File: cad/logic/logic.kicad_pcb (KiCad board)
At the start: 2 copper layers, 93 x 60 mm, 36 parts, among them J1 Conn_01x02, J10 Conn_01x02, J2 Conn_01x02, J3 Conn_01x02, J4 Conn_01x02, J5 Conn_01x02, J6 Conn_01x02, J7 Conn_01x02, J8 Conn_01x02, J9 Conn_01x06, M3 MountingHole_3.2mm_M3_ISO7380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, U1 74HC595, U2 TPL7407LAD, U3 TPL7407LAD, U4 TPL7407LAD

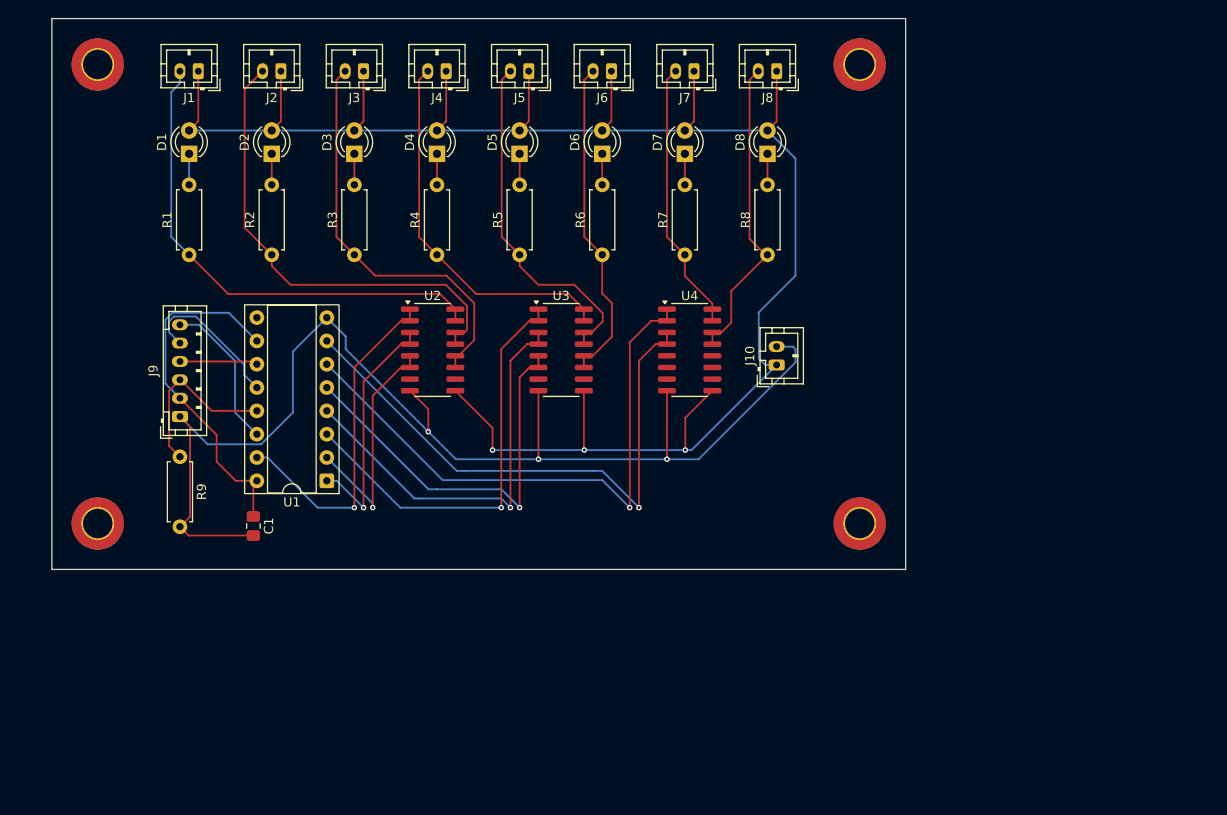
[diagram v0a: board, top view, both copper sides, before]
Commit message: Initial design complete
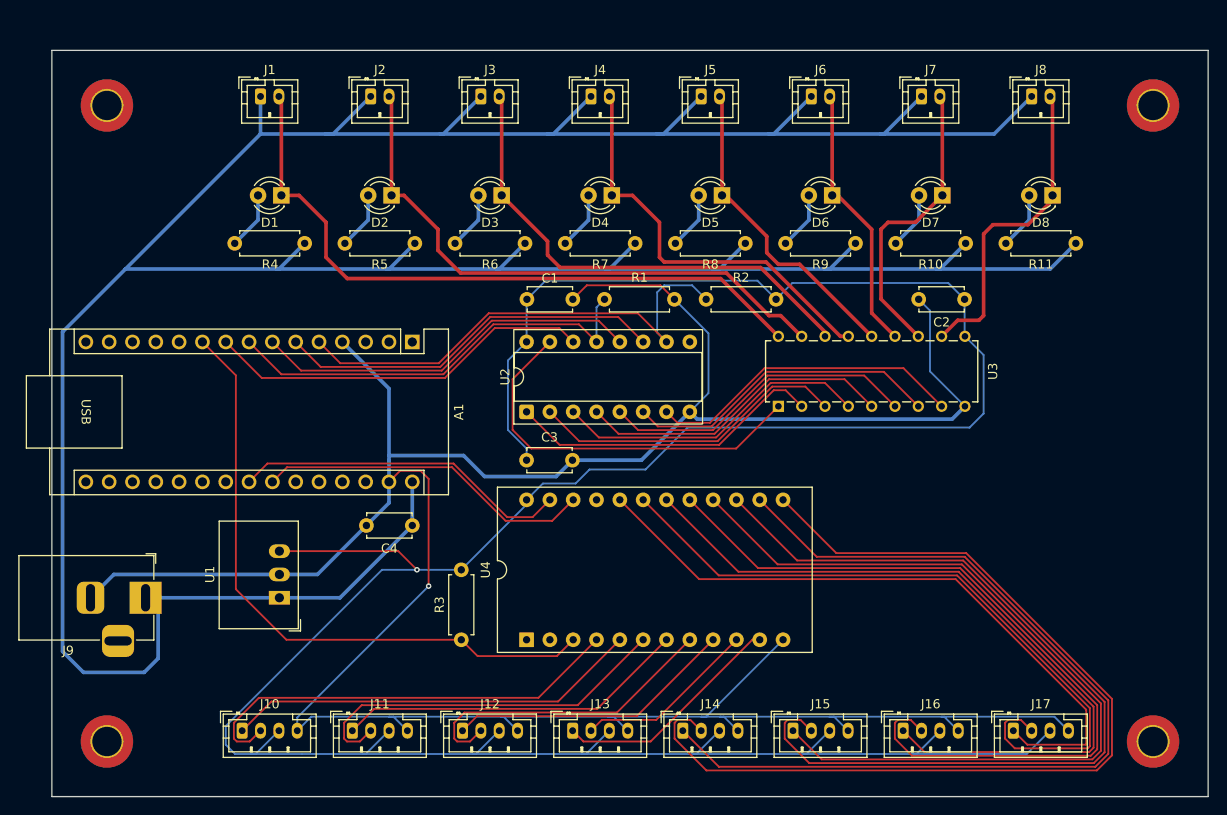
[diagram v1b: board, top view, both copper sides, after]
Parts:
- added A1: Arduino_Nano_ESP32, Module:Arduino_Nano, F.Cu at (64.3, 57.2)
- added C2: 100nF, Capacitor_THT:C_Disc_D4.7mm_W2.5mm_P5.00mm, F.Cu at (124.4, 52.6)
- added C3: 100nF, Capacitor_THT:C_Disc_D4.7mm_W2.5mm_P5.00mm, F.Cu at (76.7, 70.1)
- added C4: 100nF, Capacitor_THT:C_Disc_D4.7mm_W2.5mm_P5.00mm, F.Cu at (64.3, 77.2)
- added J11: Conn_01x04, Connector_JST:JST_PH_B4B-PH-K_1x04_P2.00mm_Vertical, F.Cu at (57.7, 99.6)
- added J12: Conn_01x04, Connector_JST:JST_PH_B4B-PH-K_1x04_P2.00mm_Vertical, F.Cu at (69.7, 99.6)
- added J13: Conn_01x04, Connector_JST:JST_PH_B4B-PH-K_1x04_P2.00mm_Vertical, F.Cu at (81.7, 99.6)
- added J14: Conn_01x04, Connector_JST:JST_PH_B4B-PH-K_1x04_P2.00mm_Vertical, F.Cu at (93.7, 99.6)
- added J15: Conn_01x04, Connector_JST:JST_PH_B4B-PH-K_1x04_P2.00mm_Vertical, F.Cu at (105.7, 99.6)
- added J16: Conn_01x04, Connector_JST:JST_PH_B4B-PH-K_1x04_P2.00mm_Vertical, F.Cu at (117.7, 99.6)
- added J17: Conn_01x04, Connector_JST:JST_PH_B4B-PH-K_1x04_P2.00mm_Vertical, F.Cu at (129.7, 99.6)
- added R10: 100R, Resistor_THT:R_Axial_DIN0207_L6.3mm_D2.5mm_P7.62mm_Horizontal, F.Cu at (116.9, 46.5)
- added R11: 100R, Resistor_THT:R_Axial_DIN0207_L6.3mm_D2.5mm_P7.62mm_Horizontal, F.Cu at (128.9, 46.5)
- C1: footprint Capacitor_SMD:C_0805_2012Metric_Pad1.18x1.45mm_HandSolder -> Capacitor_THT:C_Disc_D4.7mm_W2.5mm_P5.00mm
- J10: value Conn_01x02 -> Conn_01x04; footprint Connector_JST:JST_PH_B2B-PH-K_1x02_P2.00mm_Vertical -> Connector_JST:JST_PH_B4B-PH-K_1x04_P2.00mm_Vertical
- J9: value Conn_01x06 -> Barrel_Jack_Switch; footprint Connector_JST:JST_PH_B6B-PH-K_1x06_P2.00mm_Vertical -> Connector_BarrelJack:BarrelJack_Horizontal
- R1, R2, R3: value 1k -> 10k
- R4, R5, R6, R7, R8: value 1k -> 100R
- R9: value 10k -> 100R
- U1: value 74HC595 -> R-78E5.0-1.0; footprint Package_DIP:DIP-16_W7.62mm_Socket -> Converter_DCDC:Converter_DCDC_RECOM_R-78E-0.5_THT
- U2: value TPL7407LAD -> 74HC595; footprint Package_SO:SOIC-16_3.9x9.9mm_P1.27mm -> Package_DIP:DIP-16_W7.62mm_Socket
- U3: value TPL7407LAD -> TBD62381APG; footprint Package_SO:SOIC-16_3.9x9.9mm_P1.27mm -> footprints:P-DIP18-300-2p54-001_TOS
- U4: value TPL7407LAD -> TCA9548APWR; footprint Package_SO:SOIC-16_3.9x9.9mm_P1.27mm -> Package_DIP:DIP-24_18.0mmx34.29mm_W15.24mm_Socket
- moved M4 117.4 mm to (144.9, 100.7)
- moved M3 85.4 mm to (31.0, 100.7)
- moved J10 70.5 mm to (45.7, 99.6), turned to 0 degrees
- moved R9 69.9 mm to (104.9, 46.5), turned to 0 degrees
- moved R2 47.6 mm to (96.3, 52.6), turned to 0 degrees
- moved R1 45.5 mm to (85.2, 52.6), turned to 0 degrees
- moved R3 43.5 mm to (69.6, 89.7)
- moved C1 38.7 mm to (76.7, 52.6), turned to 0 degrees
- moved U4 36.2 mm to (76.7, 89.7), turned to 90 degrees
- moved M2 32.3 mm to (144.9, 31.5)
- moved D8 31.4 mm to (134.0, 41.3), turned to 180 degrees
- moved D7 28.4 mm to (122.0, 41.3), turned to 180 degrees
- moved J8 27.9 mm to (131.7, 30.5), turned to 0 degrees
- moved D6 25.5 mm to (110.0, 41.3), turned to 180 degrees
- moved J7 24.9 mm to (119.7, 30.5), turned to 0 degrees
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- renumbered M3 to M1, M3 to M2, M3 to M4
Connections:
- D1 pad 2: +12V -> Net-(D1-A)
- D2 pad 2: +12V -> Net-(D2-A)
- D3 pad 2: +12V -> Net-(D3-A)
- D4 pad 2: +12V -> Net-(D4-A)
- D5 pad 2: +12V -> Net-(D5-A)
- D6 pad 2: +12V -> Net-(D6-A)
- D7 pad 2: +12V -> Net-(D7-A)
- D8 pad 2: +12V -> Net-(D8-A)
- J1 pad 2: Net-(J1-Pin_2) -> Net-(D1-K)
- J10 pad 1: +12V -> Net-(J10-Pin_1)
- J10 pad 2: GND -> Net-(J10-Pin_2)
- J2 pad 2: Net-(J2-Pin_2) -> Net-(D2-K)
- J3 pad 2: Net-(J3-Pin_2) -> Net-(D3-K)
- J4 pad 2: Net-(J4-Pin_2) -> Net-(D4-K)
- J5 pad 2: Net-(J5-Pin_2) -> Net-(D5-K)
- J6 pad 2: Net-(J6-Pin_2) -> Net-(D6-K)
- J7 pad 2: Net-(J7-Pin_2) -> Net-(D7-K)
- J8 pad 2: Net-(J8-Pin_2) -> Net-(D8-K)
- J9 pad 1: GND -> +12V
- J9 pad 2: +5V -> GND
- J9 pad 3: Net-(J9-Pin_3) -> unconnected-(J9-Pad3)
- R1 pad 1: Net-(J1-Pin_2) -> Net-(A1-D5)
- R1 pad 2: Net-(D1-K) -> GND
- R2 pad 1: Net-(J2-Pin_2) -> Net-(A1-D2)
- R2 pad 2: Net-(D2-K) -> +5V
- R3 pad 1: Net-(J3-Pin_2) -> Net-(A1-D7)
- R3 pad 2: Net-(D3-K) -> +5V
- R4 pad 1: Net-(J4-Pin_2) -> Net-(D1-A)
- R4 pad 2: Net-(D4-K) -> +12V
- R5 pad 1: Net-(J5-Pin_2) -> Net-(D2-A)
- R5 pad 2: Net-(D5-K) -> +12V
- R6 pad 1: Net-(J6-Pin_2) -> Net-(D3-A)
- R6 pad 2: Net-(D6-K) -> +12V
- R7 pad 1: Net-(J7-Pin_2) -> Net-(D4-A)
- R7 pad 2: Net-(D7-K) -> +12V
- R8 pad 1: Net-(J8-Pin_2) -> Net-(D5-A)
- R8 pad 2: Net-(D8-K) -> +12V
- R9 pad 1: Net-(J9-Pin_3) -> Net-(D6-A)
- R9 pad 2: GND -> +12V
- U1 pad 1: Net-(U1-QB) -> +12V
- U1 pad 2: Net-(U1-QC) -> GND
- U1 pad 3: Net-(U1-QD) -> +5V
- U2 pad 1: Net-(U1-QA) -> Net-(U2-QB)
- U2 pad 10: unconnected-(U2-OUT7-Pad10) -> Net-(A1-D2)
- U2 pad 11: Net-(J3-Pin_2) -> Net-(A1-D3)
- U2 pad 12: Net-(J3-Pin_2) -> Net-(A1-D4)
- U2 pad 13: Net-(J2-Pin_2) -> Net-(A1-D5)
- U2 pad 14: Net-(J2-Pin_2) -> Net-(A1-D6)
- U2 pad 15: Net-(J1-Pin_2) -> Net-(U2-QA)
- U2 pad 16: Net-(J1-Pin_2) -> +5V
- U2 pad 2: Net-(U1-QA) -> Net-(U2-QC)
- U2 pad 3: Net-(U1-QB) -> Net-(U2-QD)
- U2 pad 4: Net-(U1-QB) -> Net-(U2-QE)
- U2 pad 5: Net-(U1-QC) -> Net-(U2-QF)
- U2 pad 6: Net-(U1-QC) -> Net-(U2-QG)
- U2 pad 7: unconnected-(U2-IN7-Pad7) -> Net-(U2-QH)
- U2 pad 9: +12V -> unconnected-(U2-QH&apos;-Pad9)
- U3 pad 1: Net-(U1-QD) -> Net-(U2-QA)
- U3 pad 10: unconnected-(U3-OUT7-Pad10) -> +5V
- U3 pad 11: Net-(J6-Pin_2) -> Net-(D8-K)
- U3 pad 12: Net-(J6-Pin_2) -> Net-(D7-K)
- U3 pad 13: Net-(J5-Pin_2) -> Net-(D6-K)
- U3 pad 14: Net-(J5-Pin_2) -> Net-(D5-K)
- U3 pad 15: Net-(J4-Pin_2) -> Net-(D4-K)
- U3 pad 16: Net-(J4-Pin_2) -> Net-(D3-K)
- U3 pad 2: Net-(U1-QD) -> Net-(U2-QB)
- U3 pad 3: Net-(U1-QE) -> Net-(U2-QC)
- U3 pad 4: Net-(U1-QE) -> Net-(U2-QD)
- U3 pad 5: Net-(U1-QF) -> Net-(U2-QE)
- U3 pad 6: Net-(U1-QF) -> Net-(U2-QF)
- U3 pad 7: unconnected-(U3-IN7-Pad7) -> Net-(U2-QG)
- U3 pad 8: GND -> Net-(U2-QH)
- U3 pad 9: +12V -> GND
- U4 pad 1: Net-(U1-QG) -> unconnected-(U4-A0-Pad1)
- U4 pad 10: unconnected-(U4-OUT7-Pad10) -> Net-(J13-Pin_2)
- U4 pad 11: unconnected-(U4-OUT6-Pad11) -> Net-(J13-Pin_1)
- U4 pad 12: unconnected-(U4-OUT5-Pad12) -> GND
- U4 pad 13: Net-(J8-Pin_2) -> Net-(J14-Pin_2)
- U4 pad 14: Net-(J8-Pin_2) -> Net-(J14-Pin_1)
- U4 pad 15: Net-(J7-Pin_2) -> Net-(J15-Pin_2)
- U4 pad 16: Net-(J7-Pin_2) -> Net-(J15-Pin_1)
- U4 pad 2: Net-(U1-QG) -> unconnected-(U4-A1-Pad2)
- U4 pad 3: Net-(U1-QH) -> Net-(A1-D7)
- U4 pad 4: Net-(U1-QH) -> Net-(J10-Pin_2)
- U4 pad 5: unconnected-(U4-IN5-Pad5) -> Net-(J10-Pin_1)
- U4 pad 6: unconnected-(U4-IN6-Pad6) -> Net-(J11-Pin_2)
- U4 pad 7: unconnected-(U4-IN7-Pad7) -> Net-(J11-Pin_1)
- U4 pad 8: GND -> Net-(J12-Pin_2)
- U4 pad 9: +12V -> Net-(J12-Pin_1)
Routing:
- net +5V: track 38.6 -> 317.0 mm, vias 0 -> 1
- net GND: track 134.6 -> 316.3 mm, vias 3 -> 1
- net +12V: track 205.1 -> 384.4 mm, vias 3 -> 0
- net Net-(J14-Pin_2): track 0.00 -> 106.0 mm
- net Net-(J14-Pin_1): track 0.00 -> 101.4 mm
- net Net-(J15-Pin_2): track 0.00 -> 96.4 mm
- net Net-(J15-Pin_1): track 0.00 -> 91.8 mm
- net Net-(J16-Pin_2): track 0.00 -> 86.8 mm
- net Net-(J16-Pin_1): track 0.00 -> 82.2 mm
- net Net-(J17-Pin_2): track 0.00 -> 77.2 mm
- net Net-(J17-Pin_1): track 0.00 -> 72.7 mm
- net Net-(D1-K): track 3.38 -> 73.6 mm
- net Net-(A1-D7): track 0.00 -> 68.9 mm
- net Net-(U1-QG): track 63.8 -> 0.00 mm, vias 1 -> 0
- net Net-(U1-QH): track 62.6 -> 0.00 mm, vias 1 -> 0
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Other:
- board size 93 x 60 mm -> 125.9 x 81.3 mm
